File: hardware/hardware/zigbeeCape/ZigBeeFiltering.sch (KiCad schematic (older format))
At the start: 13 parts

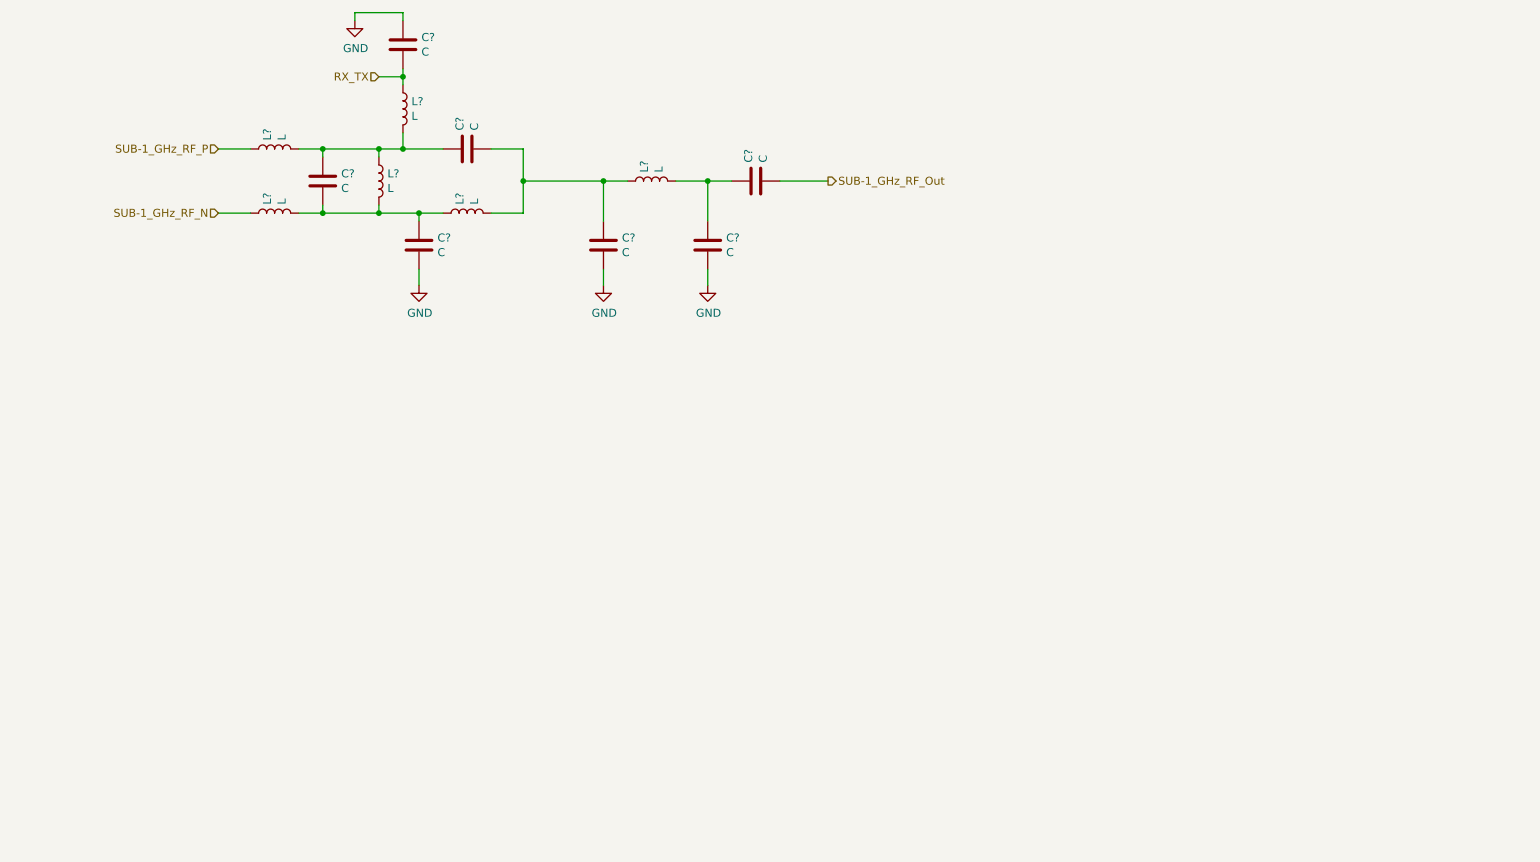
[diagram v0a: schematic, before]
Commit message: Finished Zigbee circuitry
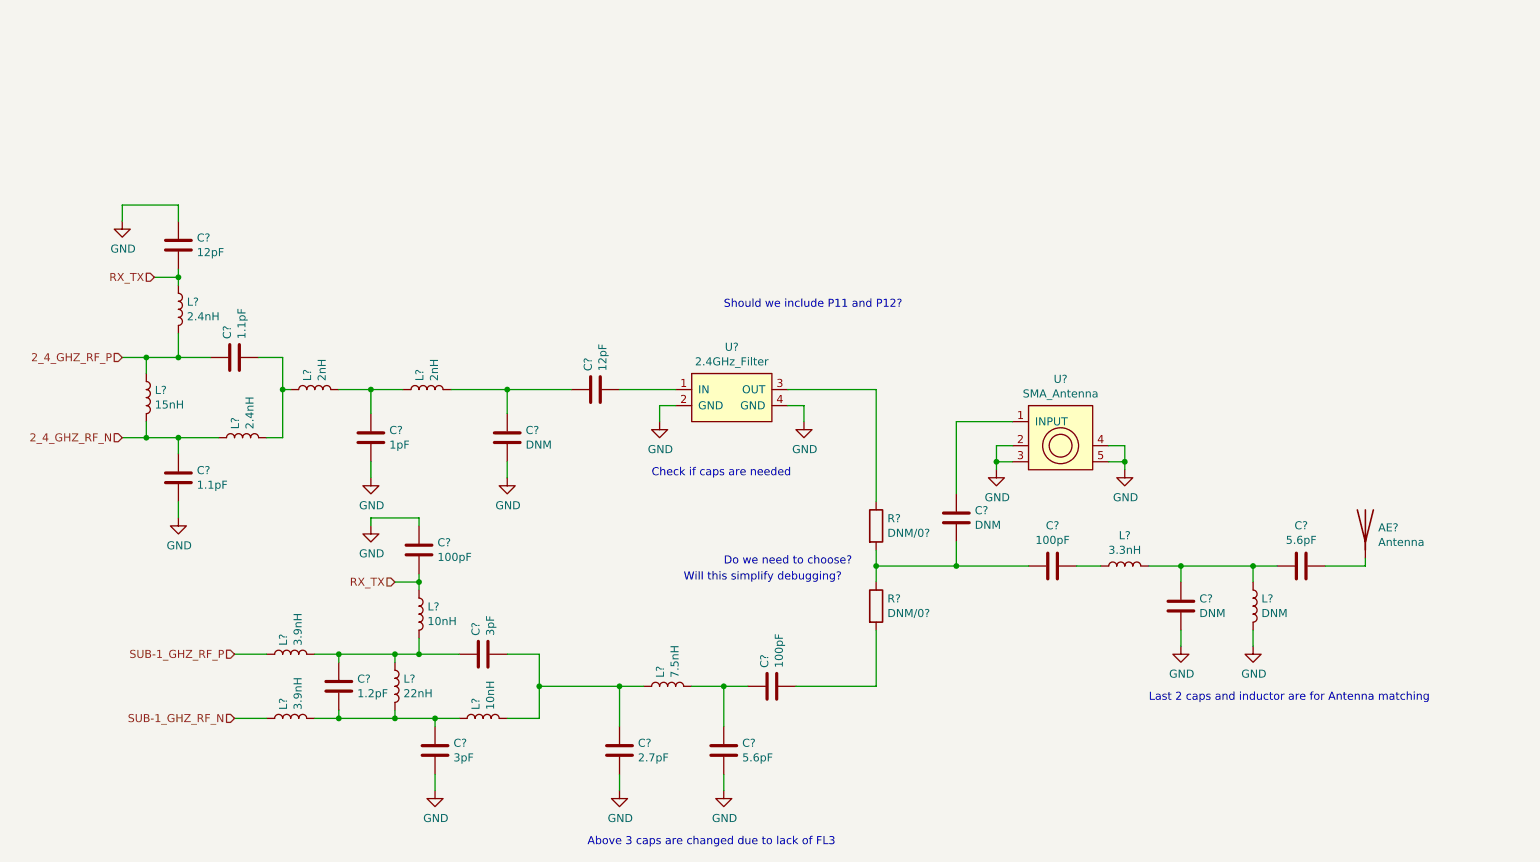
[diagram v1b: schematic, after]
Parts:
- added AE?: Antenna, symbol Device:Antenna
- added C? (x2): 1.1pF, symbol Device:C
- added C? (x2): 12pF, symbol Device:C
- added C?: 1pF, symbol Device:C
- added C? (x3): DNM, symbol Device:C
- added C?: 100pF, symbol Device:C
- added C?: 5.6pF, symbol Device:C
- added L?: 15nH, symbol Device:L
- added L? (x2): 2.4nH, symbol Device:L
- added L? (x2): 2nH, symbol Device:L
- added L?: 3.3nH, symbol Device:L
- added L?: DNM, symbol Device:L
- added R? (x2): DNM/0?, symbol Device:R
- added U?: 2.4GHz_Filter, symbol Zigbee:2.4GHz_Filter
- added U?: SMA_Antenna, symbol Zigbee:SMA_Antenna
- C? (x2): value C -> 3pF
- C? (x2): value C -> 100pF
- C?: value C -> 2.7pF
- C?: value C -> 5.6pF
- C?: value C -> 1.2pF
- L? (x2): value L -> 3.9nH
- L? (x2): value L -> 10nH
- L?: value L -> 7.5nH
- L?: value L -> 22nH
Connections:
- net GND: now also C?.1, C?.2, C?.2, C?.2, C?.2, L?.2, U?.2, U?.2 (GND), U?.3, U?.4, U?.4 (GND), U?.5
- net RX_TX: now also C?.2, L?.1
- net SUB-1_GHz_RF_N renamed SUB-1_GHZ_RF_N
- net SUB-1_GHz_RF_Out: no longer names the net of C?.2
- net SUB-1_GHz_RF_Out: now also R?.2
- net SUB-1_GHz_RF_P renamed SUB-1_GHZ_RF_P
- new net: C?.2, L?.1, L?.2
- new net: C?.1, L?.1, L?.2
- new net: C?.1, C?.1, L?.2
- new net: C?.2, U?.1 (IN)
- new net: R?.1, U?.3 (OUT)
- new net: C?.1, U?.1 (INPUT)
- new net: C?.2, C?.2, R?.1, R?.2
- new net: C?.1, L?.1
- new net: C?.1, C?.1, L?.1, L?.2
- new net: AE?.1 (A), C?.2
- new net 2_4_GHZ_RF_N: C?.1, L?.1, L?.2
- new net 2_4_GHZ_RF_P: C?.1, L?.1, L?.2
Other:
- note added: "Above 3 caps are changed due to lack of FL3"
- note added: "Check if caps are needed"
- note added: "Do we need to choose?"
- note added: "Last 2 caps and inductor are for Antenna matching\n"
- note added: "Should we include P11 and P12?"
- note added: "Will this simplify debugging?"
- moved on the sheet: C?, L?
